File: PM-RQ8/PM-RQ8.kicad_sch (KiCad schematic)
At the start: 36 parts, among them J10 2EDGR-5.08-18P, J100 2EDGK-5.08-02P, J18 2EDGK-5.08-02P, J2 PinHeader_01x05_P2.54_THT_ang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, J20 2EDGK-5.08-02P, J3 2EDGK-5.08-02P, J4 2EDGK-5.08-02P, J5 2EDGK-5.08-02P, J6 2EDGK-5.08-02P, J7 2EDGK-5.08-02P, J8 2EDGK-5.08-02P, K1 G5NB-1A-E-DC5, K2 G5NB-1A-E-DC5, K3 G5NB-1A-E-DC5, K4 G5NB-1A-E-DC5, K5 G5NB-1A-E-DC5, K6 G5NB-1A-E-DC5, K7 G5NB-1A-E-DC5, K8 G5NB-1A-E-DC5, U1 ULN2803A, U2 PCA9555PW, U4 TXS0108EPW, U5 TXB0104D

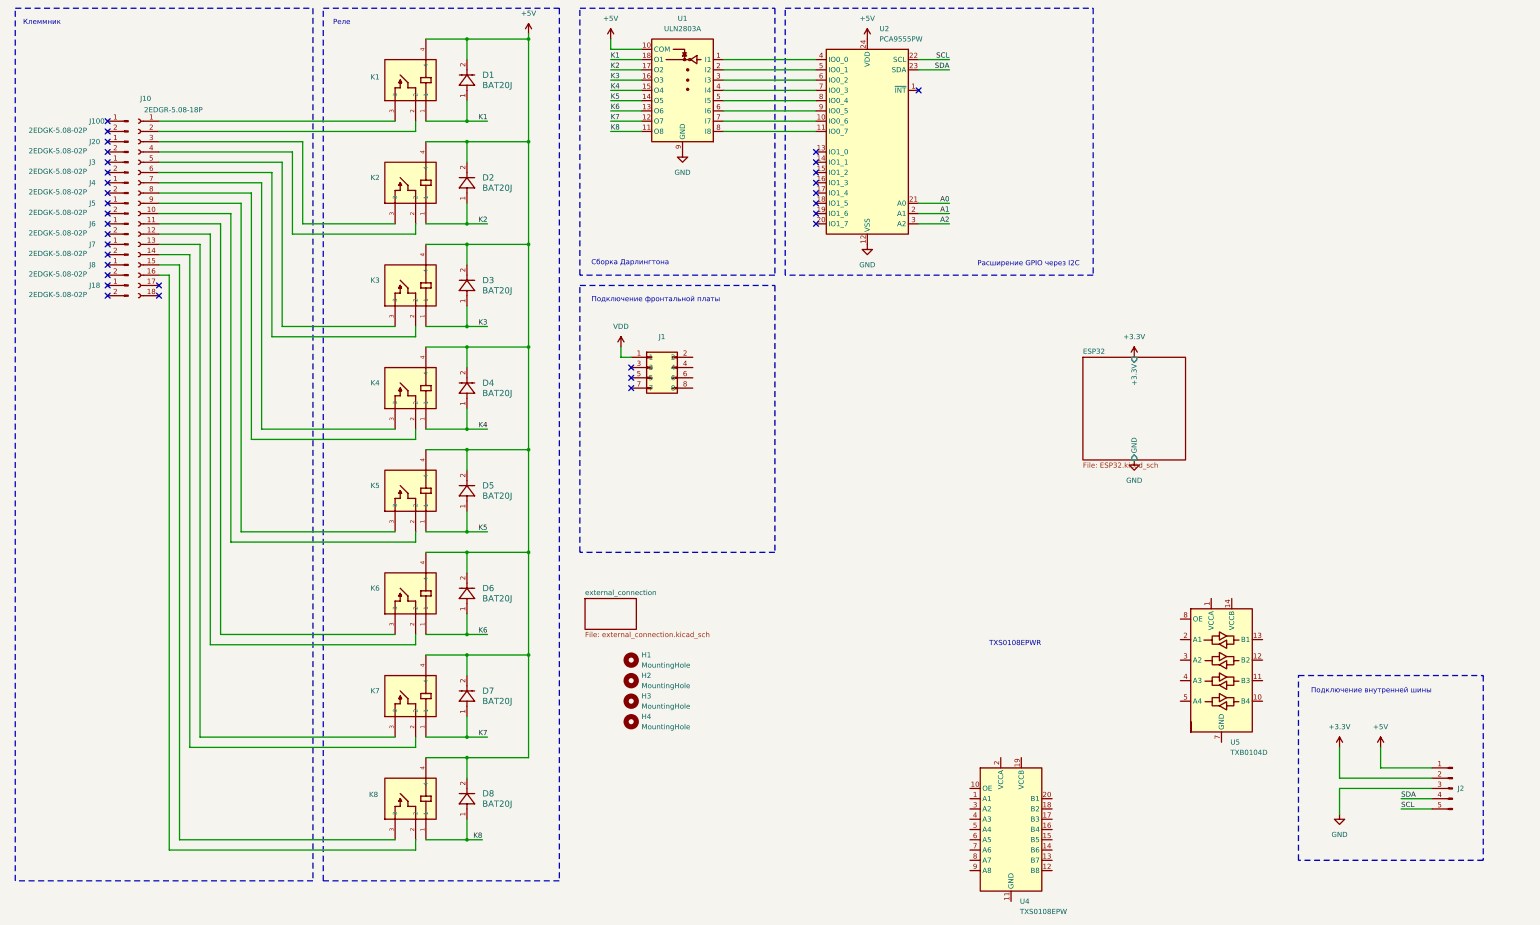
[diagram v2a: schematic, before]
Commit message: PM-RQ8
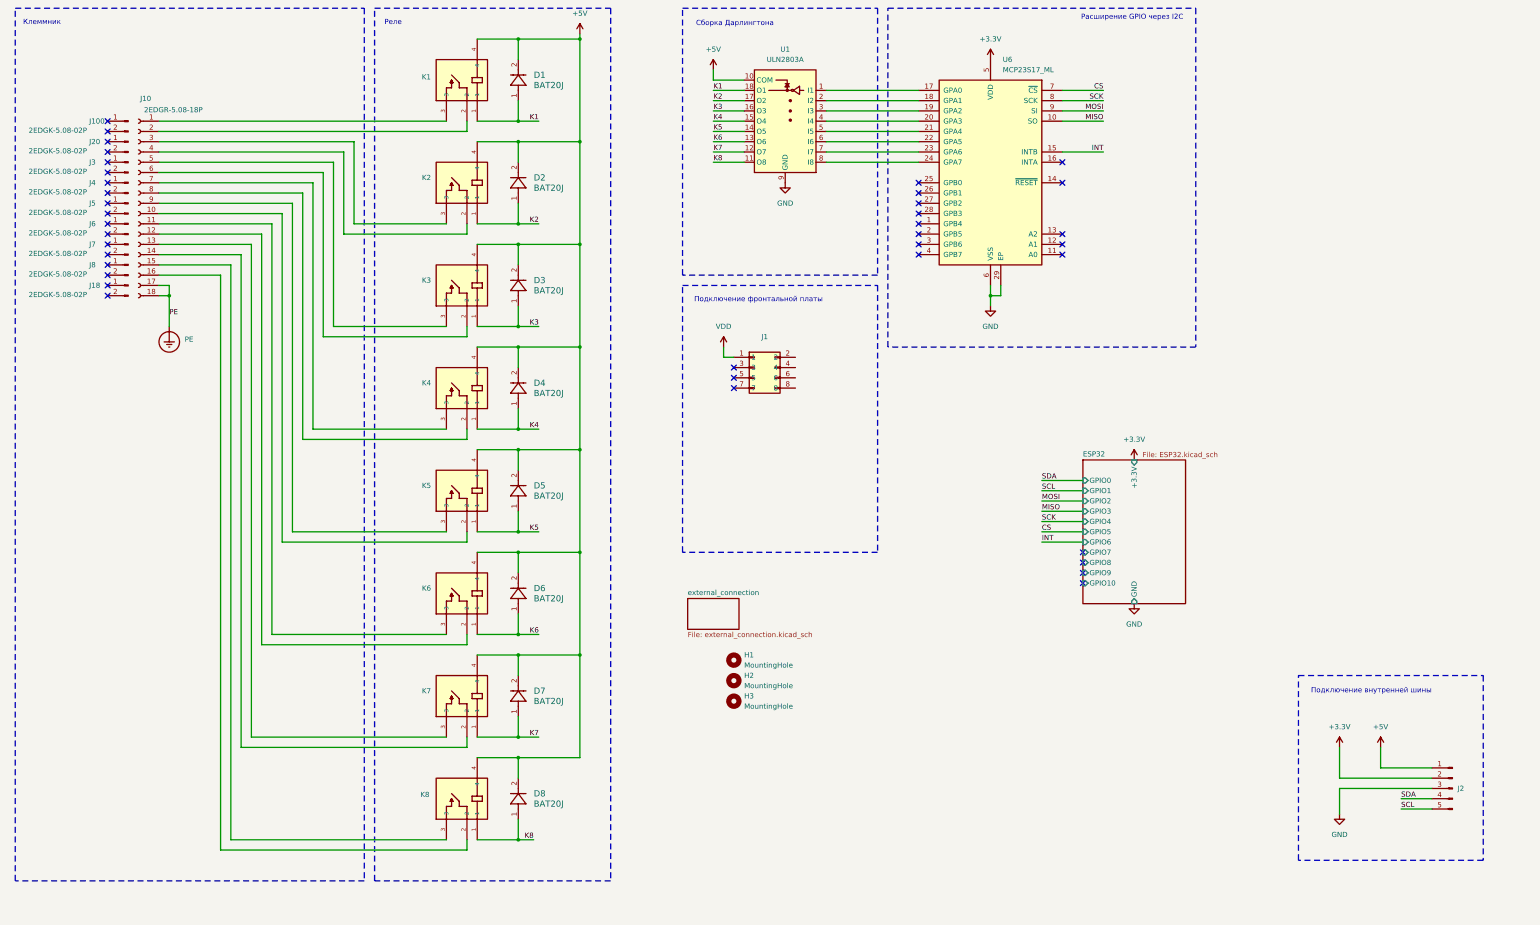
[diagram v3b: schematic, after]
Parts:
- removed H4: MountingHole, MountingHole:MountingHole_3.2mm_M3, symbol Mechanical:MountingHole
- removed U2: PCA9555PW, Package_SO:TSSOP-24_4.4x7.8mm_P0.65mm, symbol kicad_inventree_lib:PCA9555PW
- removed U4: TXS0108EPW, Package_SO:TSSOP-20_4.4x6.5mm_P0.65mm, symbol Logic_LevelTranslator:TXS0108EPW
- removed U5: TXB0104D, Package_SO:SOIC-14_3.9x8.7mm_P1.27mm, symbol Logic_LevelTranslator:TXB0104D
- added PE1: PE, kicad_inventree_lib:PE, symbol kicad_inventree_lib:PE
- added U6: MCP23S17_ML, Package_DFN_QFN:QFN-28-1EP_6x6mm_P0.65mm_EP4.25x4.25mm, symbol kicad_inventree_lib:MCP23S17_ML
- K1, K2, K3, K4, K5, K6, K7, K8: footprint NextPCB:G5NB-1A-E_DC12_RELAY_G5NB-1A_DC5_OMR -> kicad_inventree_lib:G5NB-1A-E_DC12_RELAY_G5NB-1A_DC5_OMR
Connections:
- net +3.3V: now also U6.5 (VDD)
- net GND: now also U6.29 (EP), U6.6 (VSS)
- net at U1.1 (I1): now also U6.17 (GPA0)
- net at U1.2 (I2): now also U6.18 (GPA1)
- net at U1.3 (I3): now also U6.19 (GPA2)
- net at U1.4 (I4): now also U6.20 (GPA3)
- net at U1.5 (I5): now also U6.21 (GPA4)
- net at U1.6 (I6): now also U6.22 (GPA5)
- net at U1.7 (I7): now also U6.23 (GPA6)
- net at U1.8 (I8): now also U6.24 (GPA7)
- net PE: now reaches J10.17 (Pin_17)
- net PE: now also J10.18 (Pin_18), PE1.1
- new net CS: U6.7 (~{CS})
- new net INT: U6.15 (INTB)
- new net MISO: U6.10 (SO)
- new net MOSI: U6.9 (SI)
- new net SCK: U6.8 (SCK)
- no-connect marks 32 -> 38
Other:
- sheet ESP32 ports: added GPIO0, GPIO1, GPIO10, GPIO2, GPIO3, GPIO4, GPIO5, GPIO6, GPIO7, GPIO8, GPIO9; removed none
- note removed: "TXS0108EPWR"
- moved on the sheet: D1, D2, D3, D4, D5, D6, D7, D8, H1, H2, H3, J1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
